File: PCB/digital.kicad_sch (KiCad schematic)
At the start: 29 parts, among them J1 Conn_01x06, U1 ESP32-S3, U2 PC817, U3 PC817, U4 ADuM1411

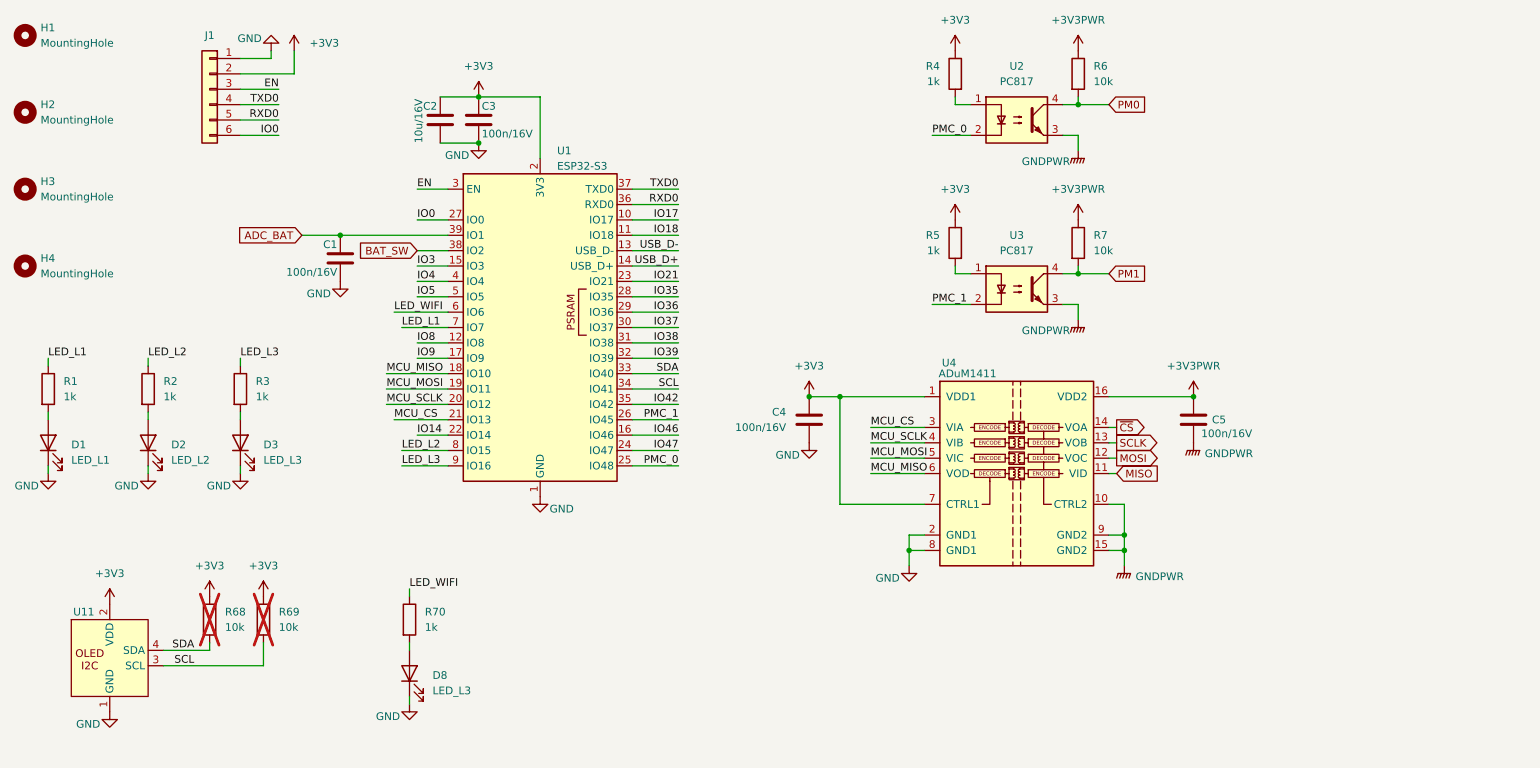
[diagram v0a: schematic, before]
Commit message: edited the PCB layout
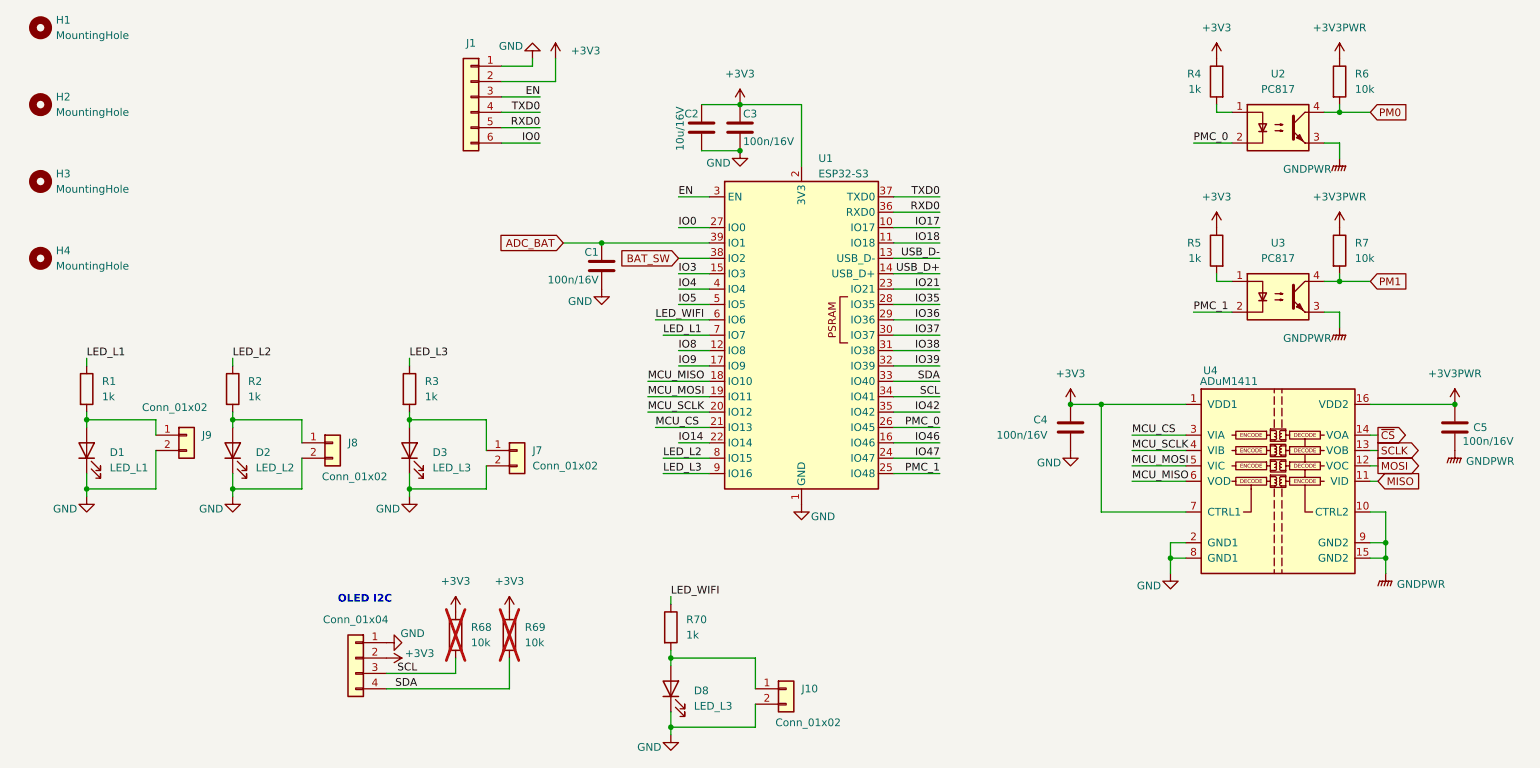
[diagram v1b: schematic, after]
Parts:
- removed U11: (no value), myLIB:128x64OLED, symbol myLIB:OLED_I2C_128x64
- added J10, J7, J8, J9: Conn_01x02, Connector_PinHeader_2.54mm:PinHeader_1x02_P2.54mm_Vertical, symbol Connector_Generic:Conn_01x02
- added J6: Conn_01x04, Connector_PinHeader_2.54mm:PinHeader_1x04_P2.54mm_Vertical, symbol Connector_Generic:Conn_01x04
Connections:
- net +3V3: now also J6.2 (Pin_2)
- net GND: now also J10.2 (Pin_2), J6.1 (Pin_1), J7.2 (Pin_2), J8.2 (Pin_2), J9.2 (Pin_2)
- net PMC_0: now also U1.26 (IO45); no longer U1.25 (IO48)
- net PMC_1: now also U1.25 (IO48); no longer U1.26 (IO45)
- net SCL: now also R68.2, J6.3 (Pin_3); no longer R69.2
- net SDA: now also R69.2, J6.4 (Pin_4); no longer R68.2
- net at D2.2 (A), R2.2: now also J8.1 (Pin_1)
- net at D3.2 (A), R3.2: now also J7.1 (Pin_1)
- net at D1.2 (A), R1.2: now also J9.1 (Pin_1)
- net at D8.2 (A), R70.2: now also J10.1 (Pin_1)
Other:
- note added: "OLED I2C"
- moved on the sheet: C1, C2, C3, C4, C5, D1, D2, D3, D8, H1, H2, H3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
